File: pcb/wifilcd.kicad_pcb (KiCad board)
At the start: 2 copper layers, 30 x 41 mm, 23 parts, among them P1 CONN_01X02, P2 CONN_01X06, Q1 BSS138, U1 AP1117D33, U2 TM022HDH26, U3 ESP-12E

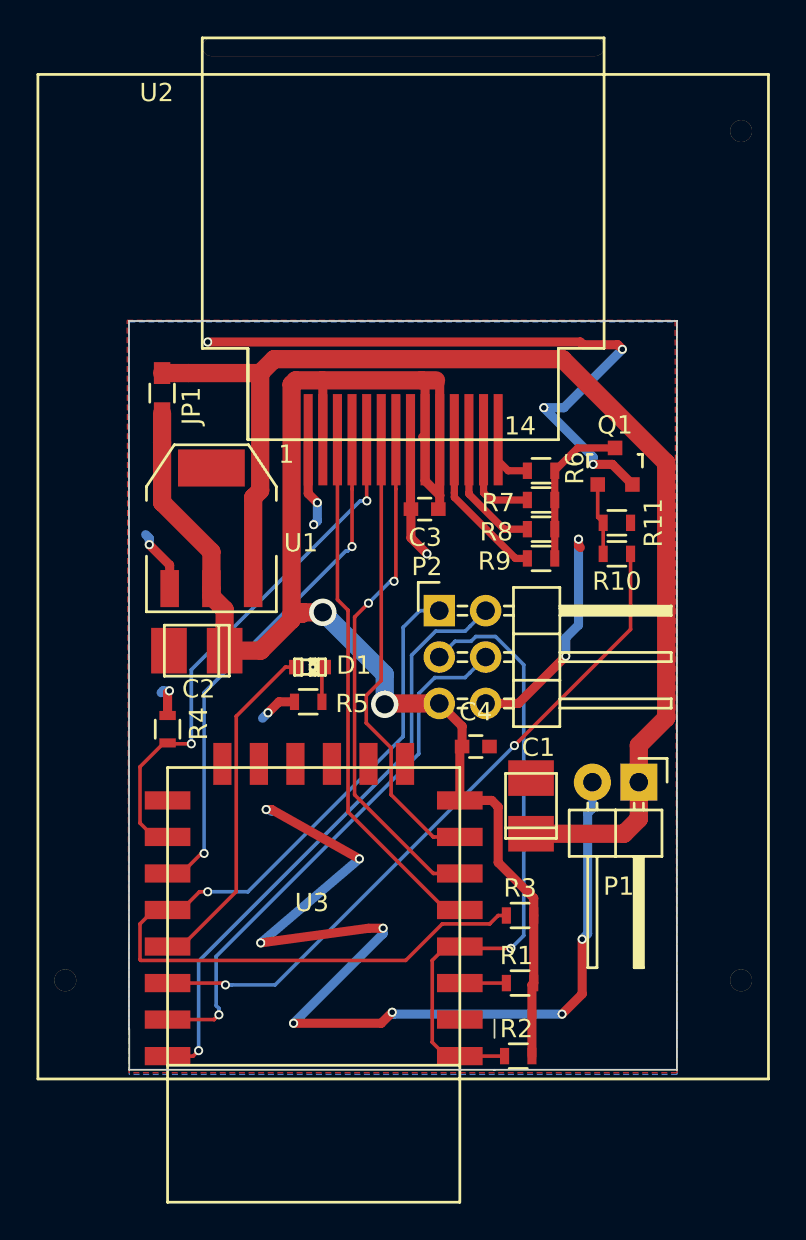
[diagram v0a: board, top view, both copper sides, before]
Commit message: Minor PCB changes
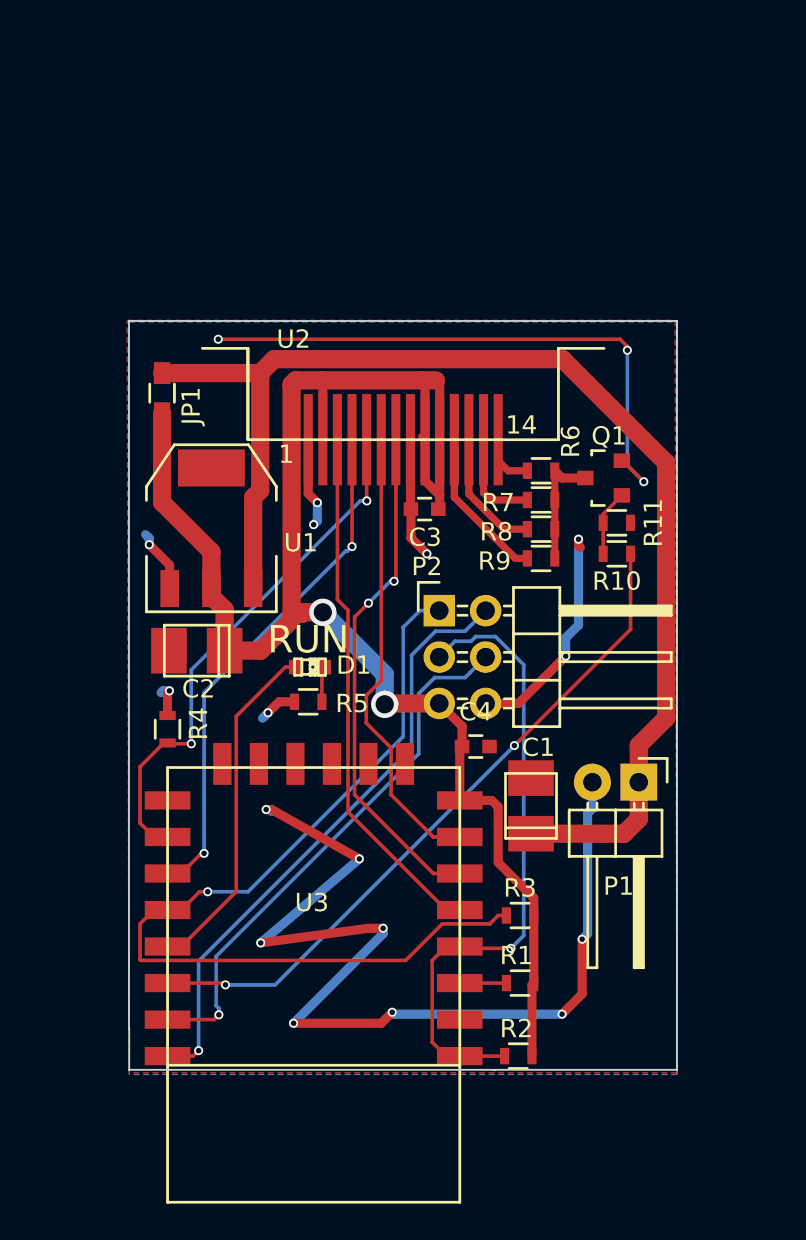
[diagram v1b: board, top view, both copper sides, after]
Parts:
- Q1: footprint Housings_SOT-23_SOT-143_TSOT-6:SOT-23 -> Housings:SOT-23
- U2: footprint Modules:TM022HDH26 -> Modules:TM022HDH26_PADSONLY
- moved Q1 0.90 mm to (97.3, 58.6), turned to 90 degrees
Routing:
- net GND: track 122.6 -> 119.3 mm, vias 20 -> 19
- net Net-(Q1-Pad3): track 8.62 -> 6.64 mm
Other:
- outline, holes or cut-outs redrawn
- board text added: "RUN"
